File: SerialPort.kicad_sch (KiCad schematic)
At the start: 9 parts, among them J4 DB9_Male, U15 MC6850, U16 MAX232, U19 74LS92

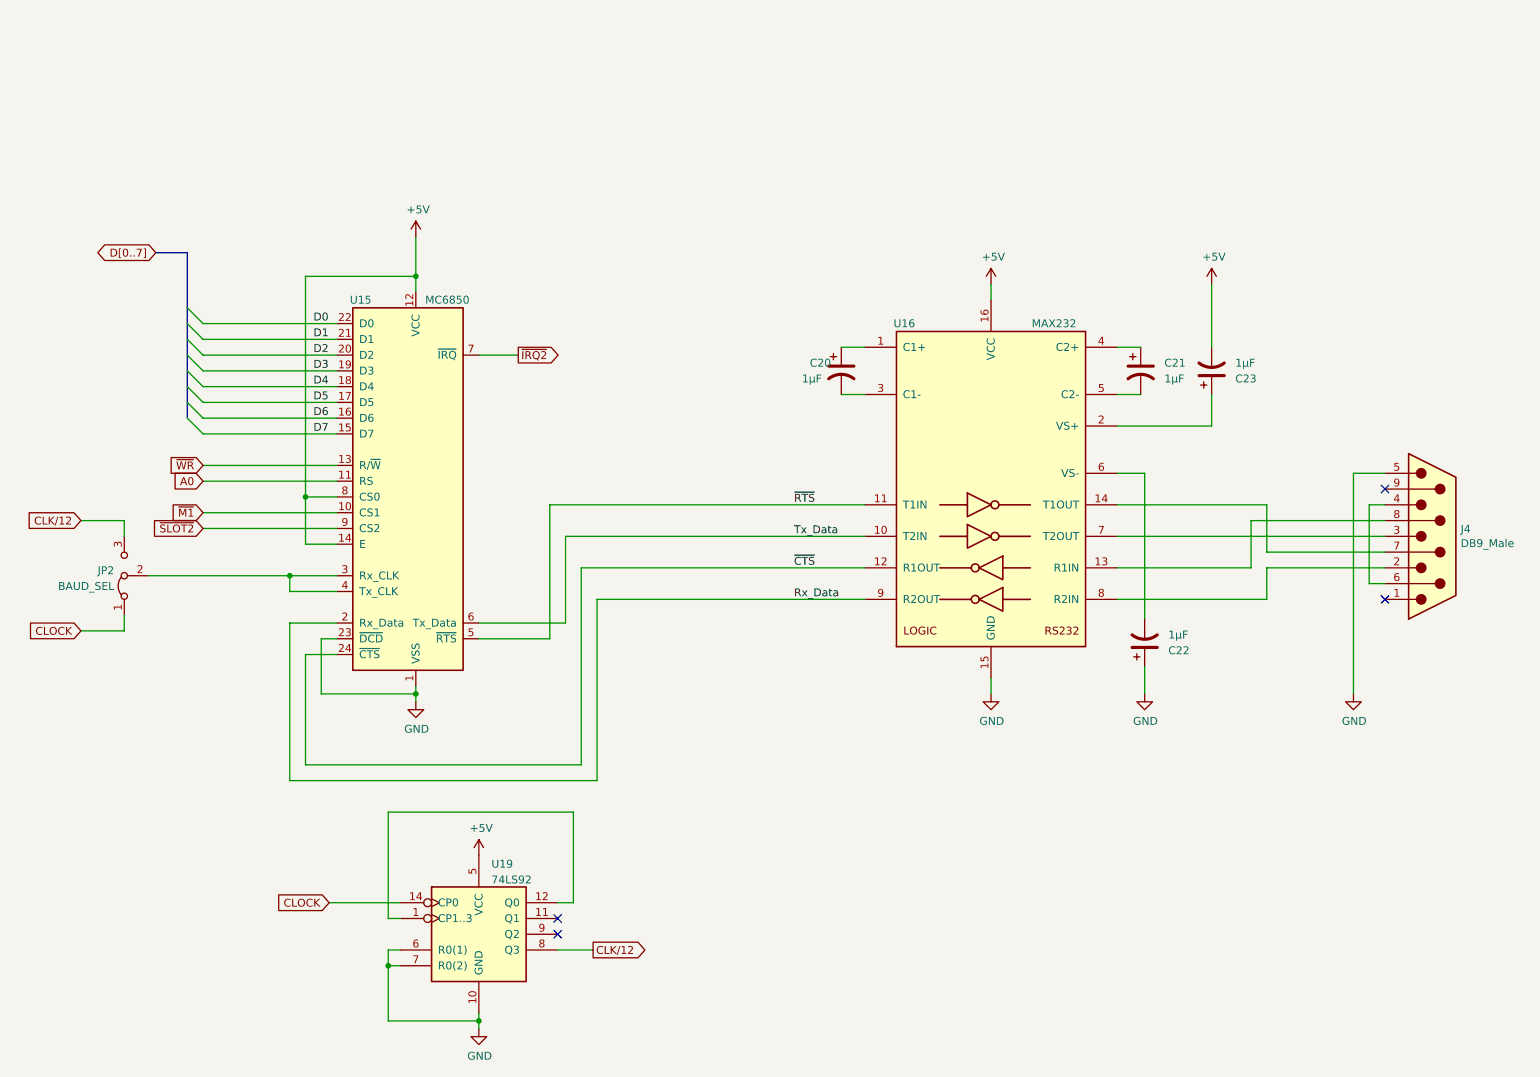
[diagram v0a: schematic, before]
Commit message: Schematic cleanup
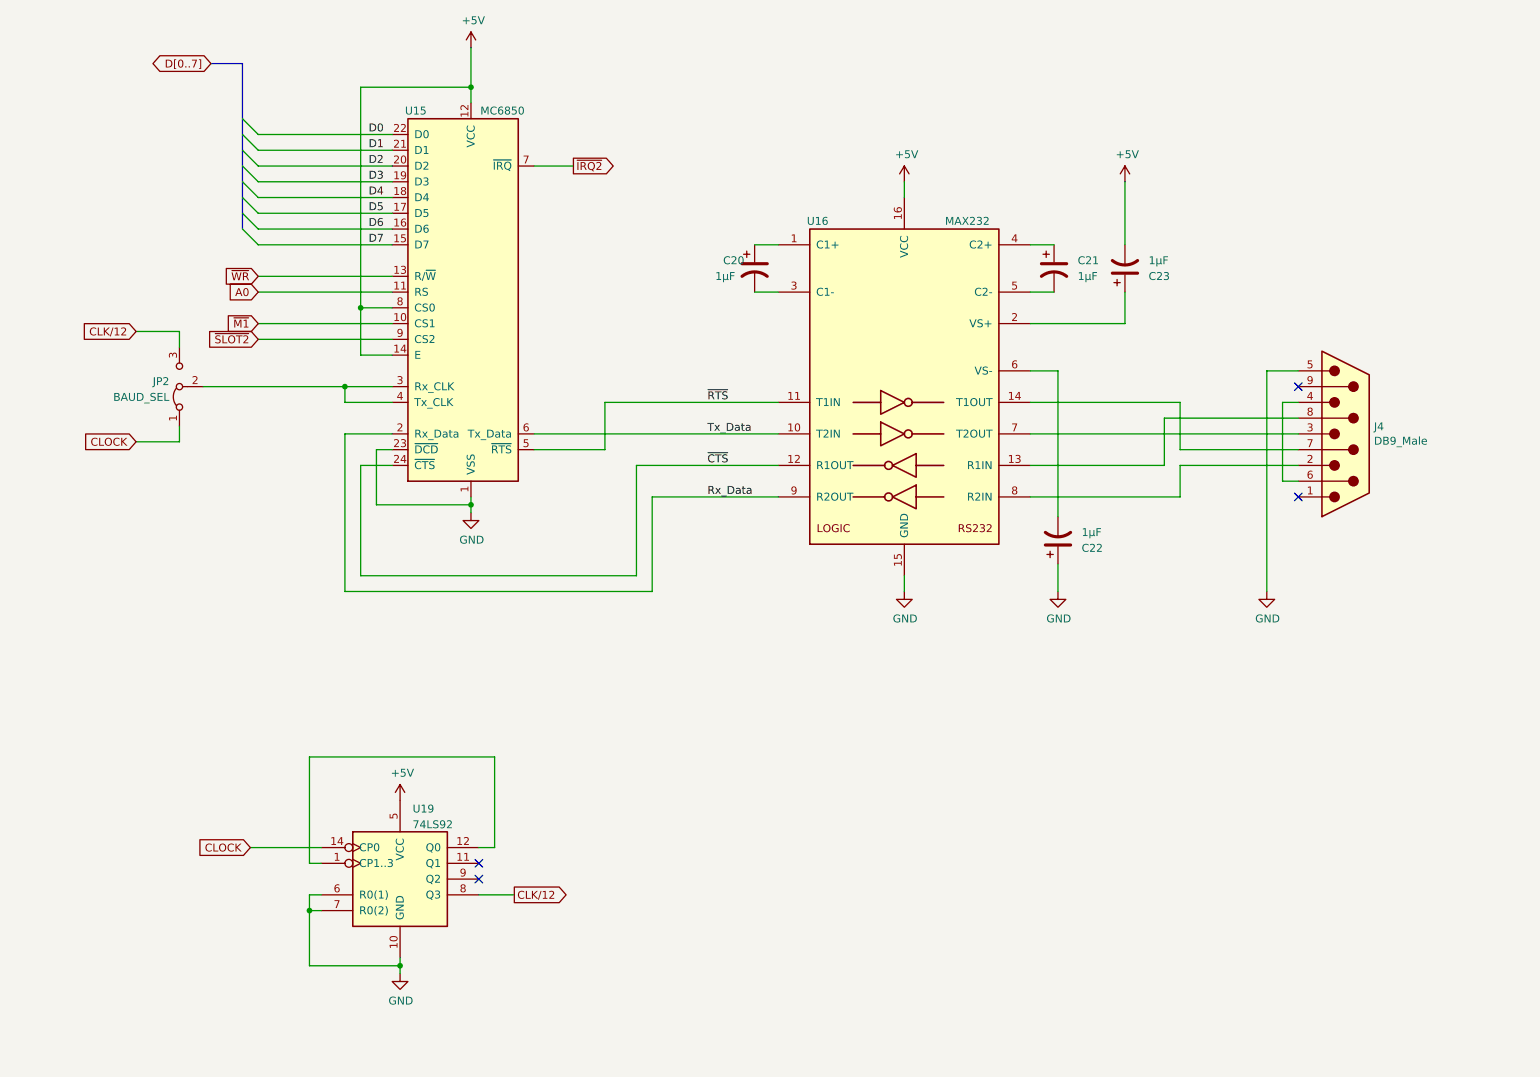
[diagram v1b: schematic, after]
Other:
- moved on the sheet: C20, C21, C22, C23, J4, JP2, U15, U16, U19

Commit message: Change serial header to shrouded
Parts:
- J4: footprint Connector_PinHeader_2.54mm:PinHeader_2x05_P2.54mm_Vertical -> Connector_IDC:IDC-Header_2x05_P2.54mm_Vertical
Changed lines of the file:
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@@
       (effects (font (size 1.27 1.27)) (justify left))
     )
-    (property "Footprint" "Connector_PinHeader_2.54mm:PinHeader_2x05_P2.54mm_Vertical" (at 229.235 98.425 0)
+    (property "Footprint" "Connector_IDC:IDC-Header_2x05_P2.54mm_Vertical" (at 229.235 98.425 0)
       (effects (font (size 1.27 1.27)) hide)
     )
